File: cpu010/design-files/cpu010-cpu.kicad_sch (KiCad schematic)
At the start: 1 part, among them U201 MC68010P

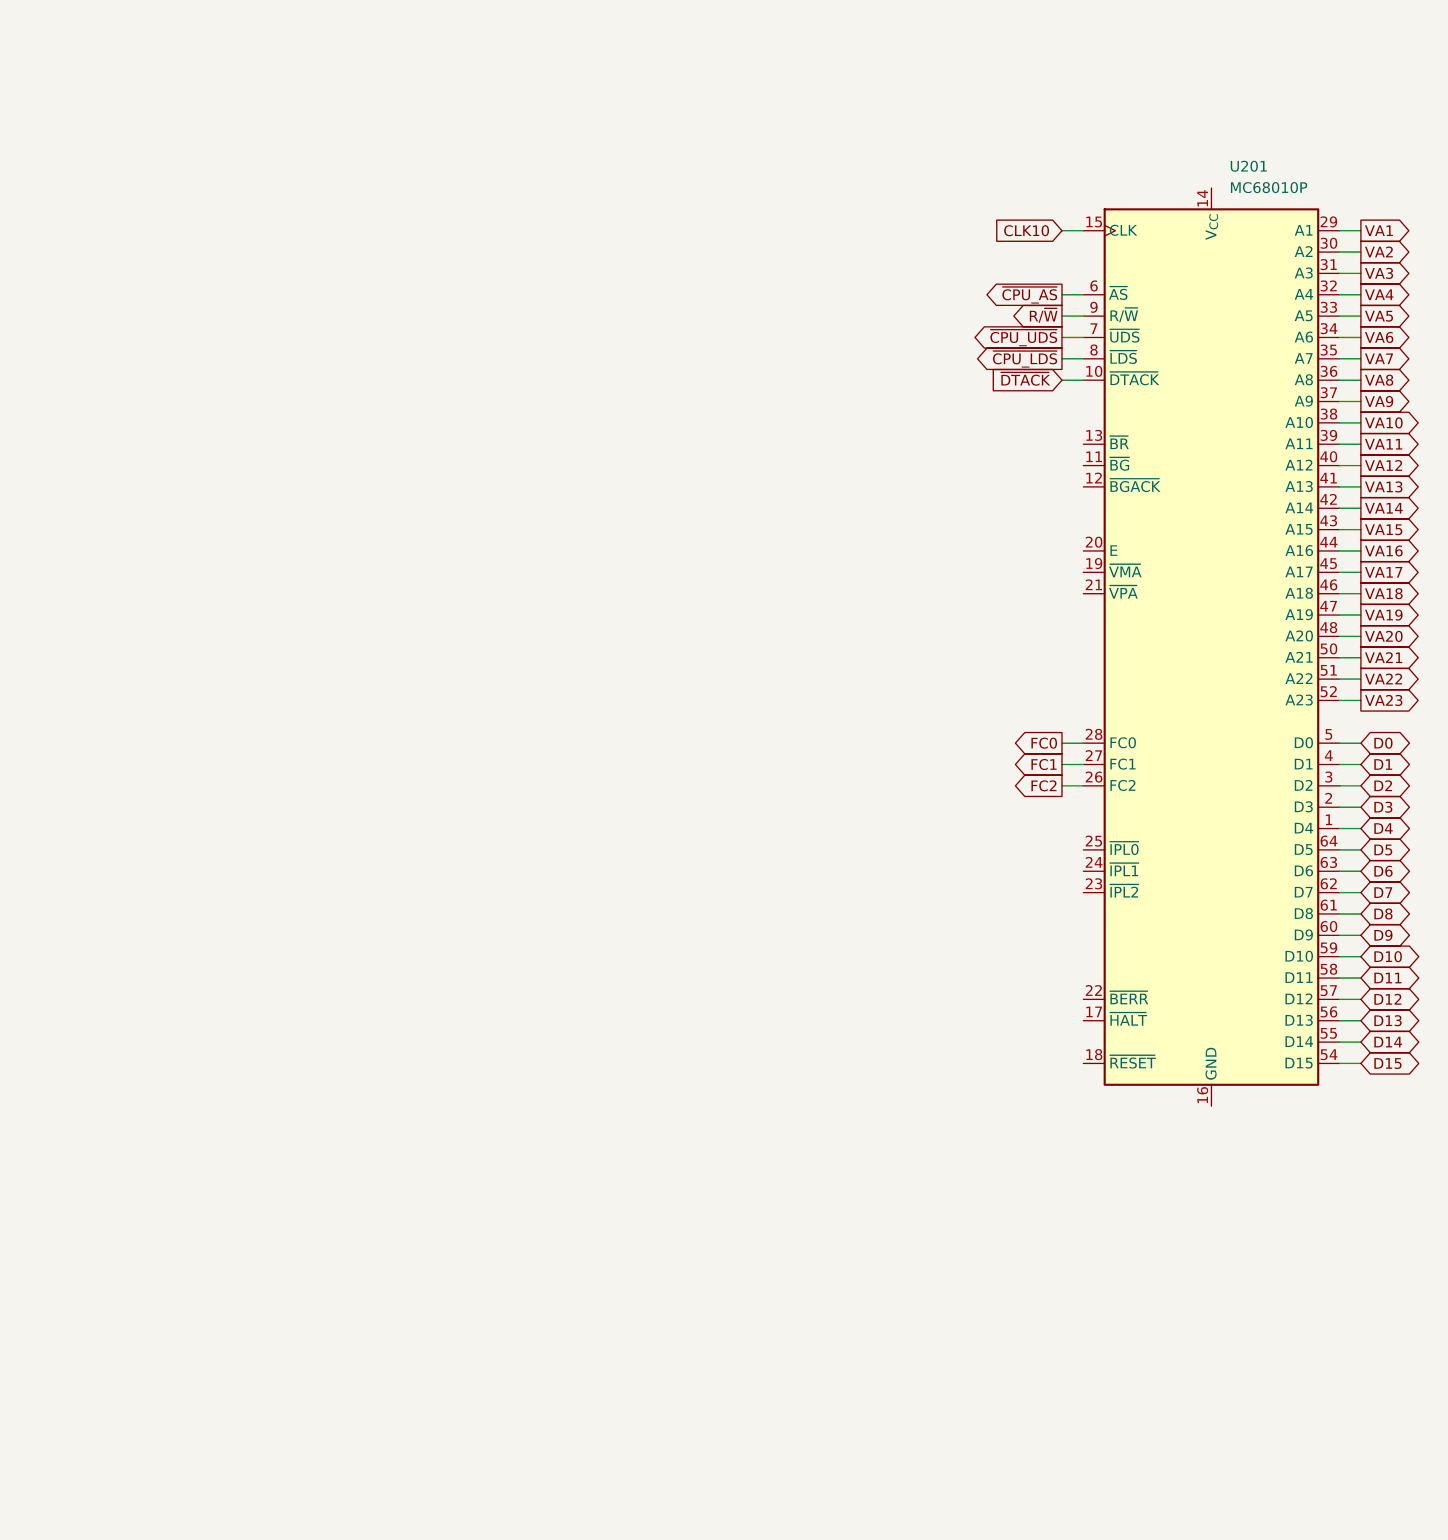
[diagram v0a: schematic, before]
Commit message: Add clock generator.
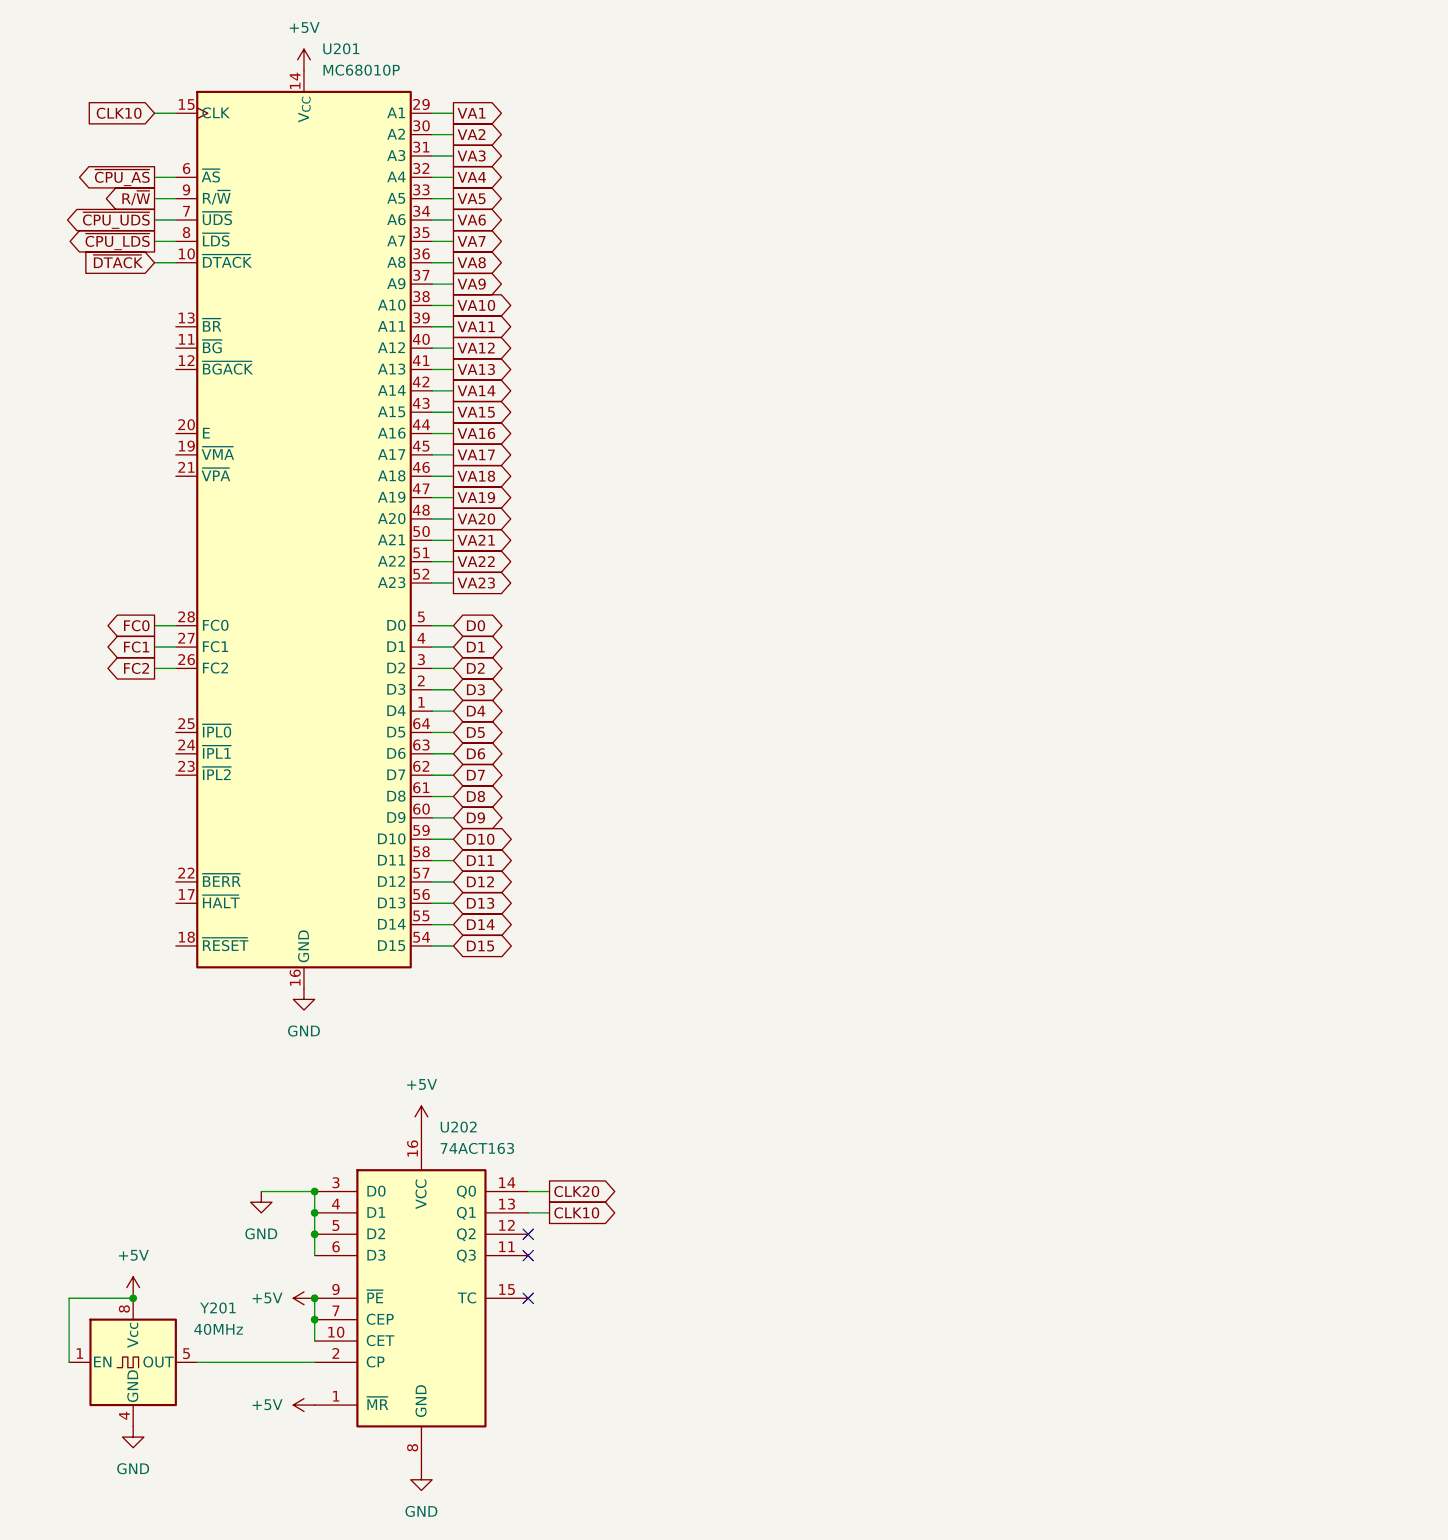
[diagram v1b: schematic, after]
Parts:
- added U202: 74ACT163, Package_DIP:DIP-16_W7.62mm_Socket, symbol 74xx:74LS163
- added Y201: 40MHz, Oscillator:Oscillator_DIP-8, symbol Oscillator:CXO_DIP8
- U201: footprint Package_DIP:DIP-64_W22.86mm -> Package_DIP:DIP-64_W22.86mm_Socket
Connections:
- net CLK10: now also U202.13 (Q1)
- net +5V: now reaches U201.14 (V_{CC}), U201.49 (V_{CC})
- net +5V: now also U202.1 (~{MR}), U202.10 (CET), U202.16 (VCC), U202.7 (CEP), U202.9 (~{PE}), Y201.1 (EN), Y201.8 (Vcc)
- net GND: now reaches U201.16 (GND), U201.53 (GND)
- net GND: now also U202.3 (D0), U202.4 (D1), U202.5 (D2), U202.6 (D3), U202.8 (GND), Y201.4 (GND)
- new net: U202.2 (CP), Y201.5 (OUT)
- new net CLK20: U202.14 (Q0)
- no-connect marks 0 -> 3
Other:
- moved on the sheet: U201
